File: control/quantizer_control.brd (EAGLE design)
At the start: 108 x 40 mm, 111 parts, among them IC1 74HC595D, IC2 74HC595D

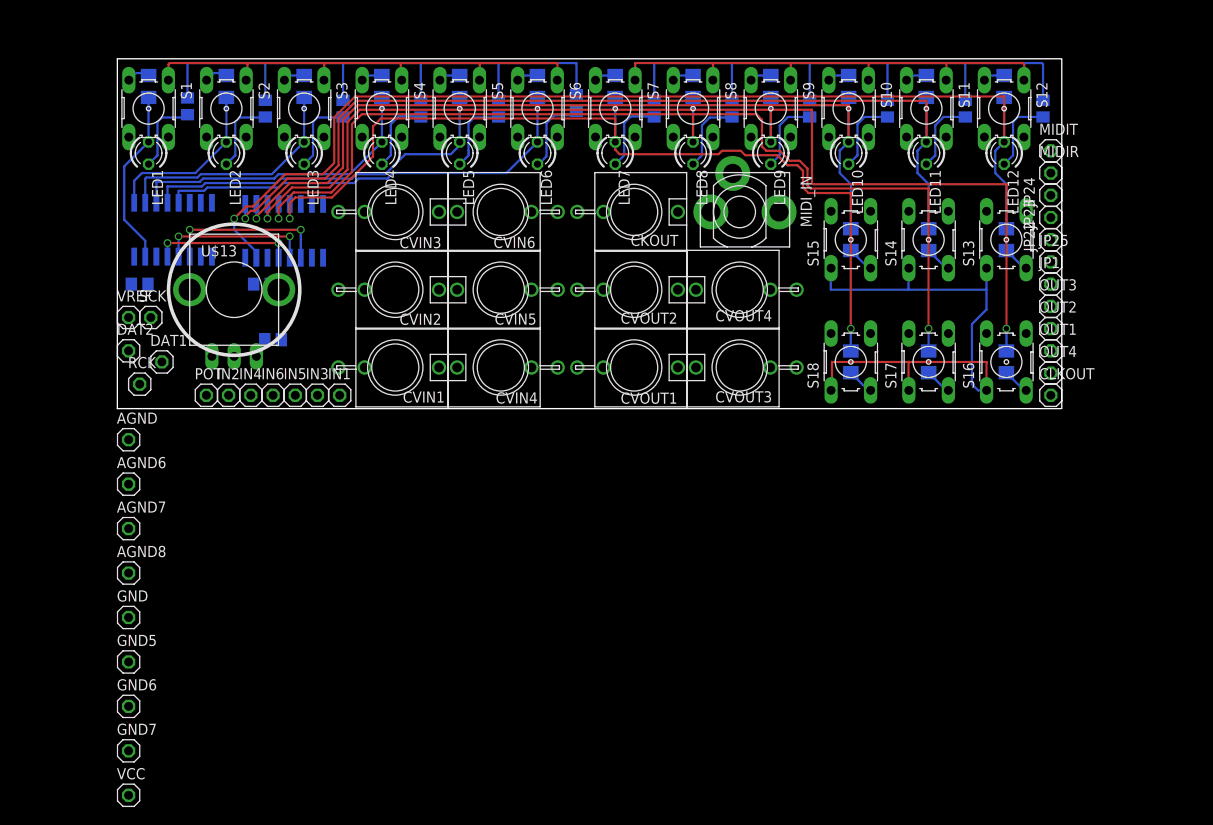
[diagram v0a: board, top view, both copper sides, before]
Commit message: SAD
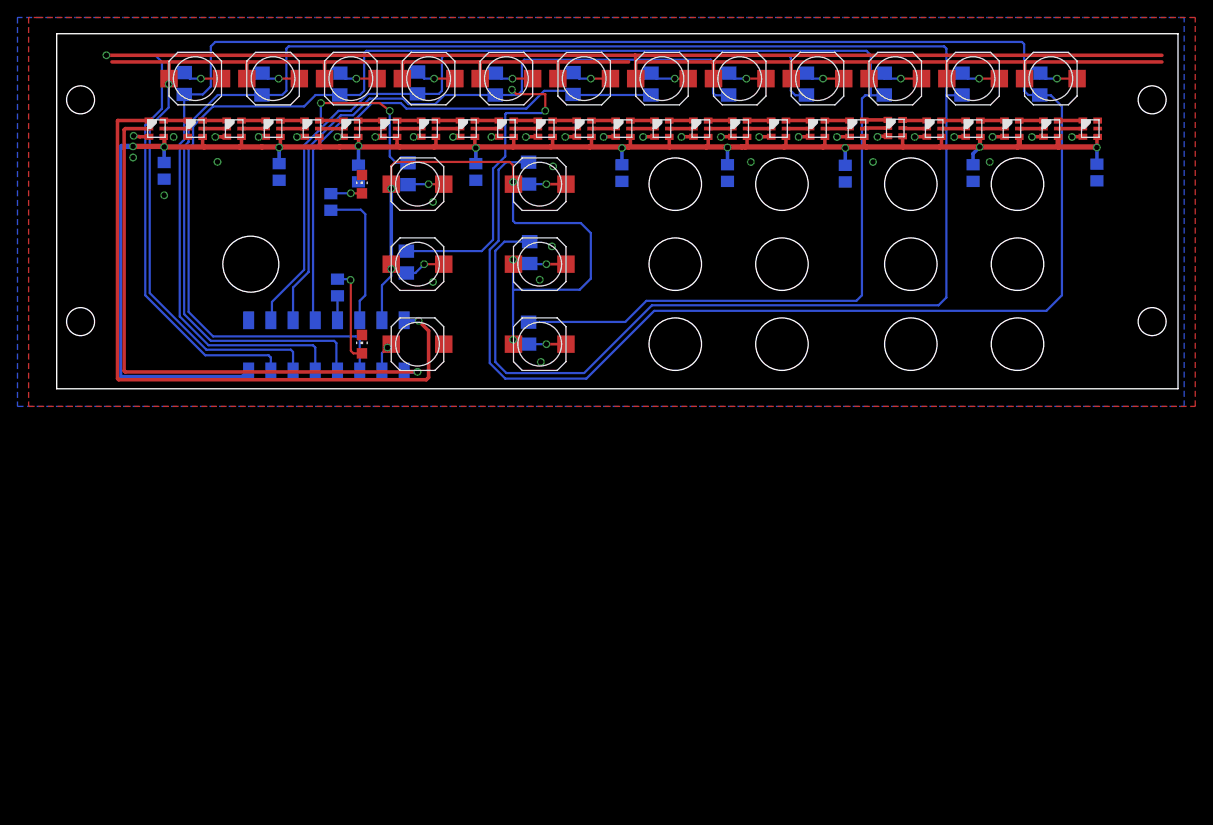
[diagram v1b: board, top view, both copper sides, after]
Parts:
- removed AGND, AGND6, AGND7, AGND8, CLKOUT, DAT1, DAT2, GND, GND5, GND6, GND7, IN1, IN2, IN3, IN4, IN5, IN6, JP1, JP22, JP23, JP24, JP25, MIDIR, MIDIT, OUT1, OUT2, OUT3, OUT4, POT, RCK, SCK, VCC, VREF: (no value), pinhead:1X01
- removed CKOUT, CVIN1, CVIN2, CVIN3, CVIN4, CVIN5, CVIN6, CVOUT1, CVOUT2, CVOUT3, CVOUT4: WQP-PJ301M-12_JACK, thonkiconn:WQP-PJ301M-12_JACK
- removed IC1, IC2: 74HC595D, 74xx-eu:SO16
- removed LED10, LED11, LED12, LED3, LED4, LED5, LED6, LED7, LED8, LED9: (no value), led:LED3MM
- removed MIDI_IN: VERTICAL_3_5MM_SOCKETTHONK, jason_eagle6:PJ301CM
- removed R10, R11, R12, R3, R4, R5, R6, R7, R8, R9: (no value), rcl:R0805
- removed S1, S10, S11, S12, S13, S14, S15, S16, S17, S18, S2, S3, S4, S5, S6, S7, S8, S9: (no value), switch-omron:B3F-10XX
- removed U$12, U$28, U$29, U$30: 0805DIODE, jasons_stuff:0805DIODE
- added C4, C5, C6, C7, C8, C9: (no value), rcl:C0805
- added D1, D10, D11, D12, D13, D14, D15, D16, D17, D2, D3, D4, D5, D6, D7, D8, D9: 0805DIODE, jasons_stuff:0805DIODE
- added SW1, SW10, SW11, SW12, SW13, SW14, SW15, SW16, SW17, SW18, SW2, SW3, SW4, SW5, SW6, SW7, SW8, SW9: SKPMSWITCH, jason_eagle6:SKPMSWITCH
- added U$1: 2X8SMT, jason_eagle6:2X8-SMT
- added U$10, U$11, U$2, U$3, U$4, U$5, U$6, U$7, U$8, U$9: APA102-2020, jason_eagle6:APA102-2020
- LED1, LED2: device led:LED3MM -> led:CHIP-LED0805
- U$13: value ALPS_POT_SMALL -> APA102-2020; device jasons_stuff:SMALL_ALPS_POT -> jason_eagle6:APA102-2020
- U$14, U$15, U$16, U$17, U$18, U$19, U$20, U$21, U$22, U$23, U$24, U$25, U$26, U$27: value 0805DIODE -> APA102-2020; device jasons_stuff:0805DIODE -> jason_eagle6:APA102-2020
- moved U$14 41.2 mm to (54.6, 34.3), flipped to the top, turned to 0 degrees
- moved U$13 40.0 mm to (50.2, 34.3)
- moved U$15 36.8 mm to (59.1, 34.3), flipped to the top, turned to 0 degrees
- moved LED1 32.7 mm to (29.2, 9.65), turned to 0 degrees
- moved U$25 32.4 mm to (103.5, 34.3), flipped to the top, turned to 0 degrees
- moved U$16 32.4 mm to (63.5, 34.3), flipped to the top, turned to 0 degrees
- moved U$26 30.1 mm to (108.0, 34.3), flipped to the top, turned to 0 degrees
- moved U$27 28.3 mm to (112.5, 34.3), flipped to the top, turned to 0 degrees
- moved U$17 28.0 mm to (67.9, 34.3), flipped to the top, turned to 0 degrees
- moved R1 26.9 mm to (26.4, 16.1), turned to 270 degrees
- moved U$18 23.6 mm to (72.4, 34.3), flipped to the top, turned to 0 degrees
- moved C1 23.0 mm to (6.60, 29.5), turned to 270 degrees
- moved C2 20.5 mm to (19.7, 29.3), turned to 270 degrees
- moved U$19 19.3 mm to (76.8, 34.3), flipped to the top, turned to 0 degrees
- moved C3 16.8 mm to (28.8, 29.2), turned to 270 degrees
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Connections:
- removed net AGND: AGND.1, AGND6.1, AGND7.1, AGND8.1, C1.2, CKOUT.P$3, CVIN1.P$2, CVIN1.P$3, CVIN2.P$2, CVIN2.P$3, CVIN3.P$2, CVIN3.P$3, CVIN4.P$2, CVIN4.P$3, CVIN5.P$2, CVIN5.P$3, CVIN6.P$2, CVIN6.P$3, CVOUT1.P$3, CVOUT2.P$3, CVOUT3.P$3, CVOUT4.P$3, U$13.A
- removed net N$66: IC1.12, IC2.12, RCK.1
- removed net N$67: IC1.11, IC2.11, SCK.1
- removed net N$68: DAT1.1, IC1.14
- removed net N$69: DAT2.1, IC2.14
- removed net VREF: U$13.B, VREF.1
- new net ALED_MOSI: U$1.15, U$2.1
- new net ALED_SCK: U$1.16, U$2.2
- new net CKI2: U$14.5, U$15.2
- new net COM0: SW1.P$2, SW2.P$2, SW3.P$2, SW4.P$2, SW5.P$2, SW6.P$2, U$1.6
- new net COM1: SW10.P$2, SW11.P$2, SW12.P$2, SW7.P$2, SW8.P$2, SW9.P$2, U$1.4
- new net COM2: SW13.P$2, SW14.P$2, SW15.P$2, SW16.P$2, SW17.P$2, U$1.13
- new net KEY0: D1.C, D12.C, D15.C, U$1.8
- new net KEY1: D11.C, D16.C, D2.C, U$1.10
- new net KEY2: D10.C, D17.C, D3.C, U$1.12
- new net KEY3: D13.C, D4.C, D9.C, U$1.3
- new net KEY4: D14.C, D5.C, D8.C, U$1.5
- new net KEY5: D6.C, D7.C, U$1.7
- new net LED0: R1.2, U$1.9
- new net LED1: R2.2, U$1.11
- new net N$62: D16.A, SW14.P$1
- new net N$63: D17.A, SW15.P$1
- new net N$64: D13.A, SW16.P$1
- new net N$65: D14.A, SW17.P$1
- new net SDI2: U$14.6, U$15.1
- new net SW1: SW18.P$1, U$1.14
- net GND: now also C1.2, C2.2, C3.2, C4.2, C5.2, C6.2, C7.2, C8.2, C9.2, LED1.C, LED2.C, SW18.P$2, U$1.1, U$10.3, U$11.3, U$13.3, U$14.3, U$15.3, U$16.3, U$17.3, U$18.3, U$19.3, U$2.3, U$20.3, U$21.3, U$22.3, U$23.3, U$24.3, U$25.3, U$26.3, U$27.3, U$3.3, U$4.3, U$5.3, U$6.3, U$7.3, U$8.3, U$9.3; no longer C2.1, C3.1, GND.1, GND5.1, GND6.1, GND7.1, IC1.13, IC1.8, IC2.13, IC2.8
- net N$1: now also U$26.6, U$27.1; no longer IC1.15, LED1.A, U$12.A
- net N$10: now also D6.A, SW6.P$1; no longer IC2.2, LED10.A, U$22.A, U$28.A
- net N$11: now also U$3.6, U$4.1; no longer IC2.1, LED11.A, U$23.A, U$29.A
- net N$12: now also U$3.5, U$4.2; no longer IC2.15, LED12.A, U$24.A, U$30.A
- net N$13: now also U$4.6, U$5.1; no longer LED1.K, R1.1
- net N$14: now also U$4.5, U$5.2; no longer LED2.K, R2.1
- net N$15: now also U$5.6, U$6.1; no longer LED3.K, R3.1
- net N$16: now also U$5.5, U$6.2; no longer LED4.K, R4.1
- net N$17: now also U$6.6, U$7.1; no longer LED5.K, R5.1
- net N$18: now also U$6.5, U$7.2; no longer LED6.K, R6.1
- net N$19: now also U$7.6, U$8.1; no longer LED7.K, R7.1
- net N$2: now also U$26.5, U$27.2; no longer IC1.1, LED2.A, U$14.A
- net N$20: now also U$7.5, U$8.2; no longer LED8.K, R8.1
- net N$21: now also U$8.6, U$9.1; no longer LED9.K, R9.1
- net N$22: now also U$8.5, U$9.2; no longer LED10.K, R10.1
- net N$23: now also U$10.1, U$9.6; no longer LED11.K, R11.1
- net N$24: now also U$10.2, U$9.5; no longer LED12.K, R12.1
- net N$25: now also U$10.6, U$11.1; no longer JP24.1, R1.2, R2.2, R3.2, R4.2, R5.2, R6.2
- net N$26: now also U$10.5, U$11.2; no longer JP23.1, R10.2, R11.2, R12.2, R7.2, R8.2, R9.2
- net N$27: now also U$11.6, U$13.1; no longer S6.3, U$18.C
- net N$28: now also U$11.5, U$13.2; no longer S5.3, U$17.C
- net N$29: now also U$13.6, U$14.1; no longer S4.3, U$16.C
- net N$3: now also D1.A, SW1.P$1; no longer IC1.2, LED3.A, U$15.A
- net N$30: now also D7.A, SW7.P$1; no longer S3.3, U$15.C
- net N$31: now also U$13.5, U$14.2; no longer S2.3, U$14.C
- net N$32: now also LED1.A, R1.1; no longer S1.3, U$12.C
- net N$33: now also U$15.6, U$16.1; no longer JP22.1, S1.1, S2.1, S3.1, S4.1, S5.1, S6.1
- net N$34: now also U$15.5, U$16.2; no longer S12.3, U$24.C
- net N$35: now also U$16.6, U$17.1; no longer S11.3, U$23.C
- net N$36: now also D8.A, SW8.P$1; no longer S10.3, U$22.C
- net N$37: now also U$16.5, U$17.2; no longer S9.3, U$21.C
- net N$38: now also U$17.6, U$18.1; no longer S8.3, U$20.C
- net N$39: now also U$17.5, U$18.2; no longer S7.3, U$19.C
- net N$4: now also D2.A, SW2.P$1; no longer IC1.3, LED4.A, U$16.A
- net N$40: now also U$18.6, U$19.1; no longer JP25.1, S10.1, S11.1, S12.1, S7.1, S8.1, S9.1
- net N$41: now also U$18.5, U$19.2; no longer S13.3, U$30.C
- net N$42: now also U$19.6, U$20.1; no longer S14.3, U$29.C
- net N$43: now also U$19.5, U$20.2; no longer S15.3, U$28.C
- net N$44: now also U$20.6, U$21.1; no longer S16.3, U$27.C
- net N$45: now also D9.A, SW9.P$1; no longer S17.3, U$26.C
- net N$46: now also U$20.5, U$21.2; no longer S18.3, U$25.C
- net N$47: now also U$21.6, U$22.1; no longer JP1.1, S13.1, S14.1, S15.1, S16.1, S17.1, S18.1
- net N$48: now also U$21.5, U$22.2; no longer MIDIT.1, MIDI_IN.T
- net N$49: now also D10.A, SW10.P$1; no longer CVIN6.P$1, IN6.1
- net N$5: now also D3.A, SW3.P$1; no longer IC1.4, LED5.A, U$17.A
- net N$50: now also U$22.6, U$23.1; no longer CVIN5.P$1, IN5.1
- net N$51: now also U$22.5, U$23.2; no longer CVIN4.P$1, IN4.1
- net N$52: now also U$23.6, U$24.1; no longer CVOUT3.P$1, OUT3.1
- net N$53: now also U$23.5, U$24.2; no longer CVOUT2.P$1, OUT2.1
- net N$54: now also U$24.6, U$25.1; no longer CVIN3.P$1, IN3.1
- net N$55: now also U$24.5, U$25.2; no longer CVIN2.P$1, IN2.1
- net N$56: now also U$25.6, U$26.1; no longer CVIN1.P$1, IN1.1
- net N$57: now also U$25.5, U$26.2; no longer CVOUT1.P$1, OUT1.1
- net N$58: now also LED2.A, R2.1; no longer CKOUT.P$1, CLKOUT.1
- net N$59: now also D11.A, SW11.P$1; no longer CVOUT4.P$1, OUT4.1
- net N$6: now also D4.A, SW4.P$1; no longer IC1.5, LED6.A, U$18.A
- net N$60: now also D12.A, SW12.P$1; no longer MIDIR.1, MIDI_IN.R
- net N$61: now also D15.A, SW13.P$1; no longer C1.1, POT.1, U$13.W
- net N$7: now also D5.A, SW5.P$1; no longer IC2.5, LED7.A, U$19.A, U$25.A
- net N$8: now also U$2.6, U$3.1; no longer IC2.4, LED8.A, U$20.A, U$26.A
- net N$9: now also U$2.5, U$3.2; no longer IC2.3, LED9.A, U$21.A, U$27.A
- net VCC: now also C1.1, C2.1, C3.1, C4.1, C5.1, C6.1, C7.1, C8.1, C9.1, U$1.2, U$10.4, U$11.4, U$13.4, U$14.4, U$15.4, U$16.4, U$17.4, U$18.4, U$19.4, U$2.4, U$20.4, U$21.4, U$22.4, U$23.4, U$24.4, U$25.4, U$26.4, U$27.4, U$3.4, U$4.4, U$5.4, U$6.4, U$7.4, U$8.4, U$9.4; no longer C2.2, C3.2, IC1.10, IC1.16, IC2.10, IC2.16, VCC.1
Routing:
- net KEY0: track 0.00 -> 274.9 mm
- net COM1: track 0.00 -> 248.0 mm, vias 0 -> 1
- net KEY1: track 0.00 -> 240.2 mm
- net VCC: track 0.00 -> 212.2 mm, vias 0 -> 10
- net KEY2: track 0.00 -> 199.9 mm
- net N$9: track 131.2 -> 2.75 mm, vias 3 -> 0
- net N$12: track 123.5 -> 2.75 mm, vias 1 -> 0
- net COM0: track 0.00 -> 117.6 mm, vias 0 -> 1
- net KEY4: track 0.00 -> 115.5 mm, vias 0 -> 2
- net N$8: track 118.1 -> 2.76 mm, vias 3 -> 0
- net KEY3: track 0.00 -> 108.3 mm, vias 0 -> 2
- net N$11: track 109.0 -> 2.76 mm, vias 1 -> 0
- net N$7: track 103.8 -> 4.52 mm, vias 3 -> 1
- net N$10: track 98.2 -> 4.55 mm
- net ALED_MOSI: track 0.00 -> 77.4 mm, vias 0 -> 1
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- added copper zone on layer 1, net GND
- added copper zone on layer 16, net GND
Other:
- board size 108 x 40 mm -> 128.2 x 40.6 mm
- board text added: "AMT"
- board text added: "CHRD"
- board text added: "GRID"
- board text added: "IN"
- board text added: "MIDI"
- board text added: "OUT1"
- board text added: "OUT2"
- board text added: "OUT3"
- board text added: "OUT4"
- board text added: "ROOT"
- board text added: "SAVE"
- board text added: "SCAL"
- board text added: "SHFT"
- board text added: "TRG"
